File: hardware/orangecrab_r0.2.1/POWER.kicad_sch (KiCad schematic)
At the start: 43 parts, among them J5 JST, U1 TLV62569DRL, U10 NCP115-2.5, U2 TLV62569DRL, U5 BQ24232, U7 TLV62569DRL

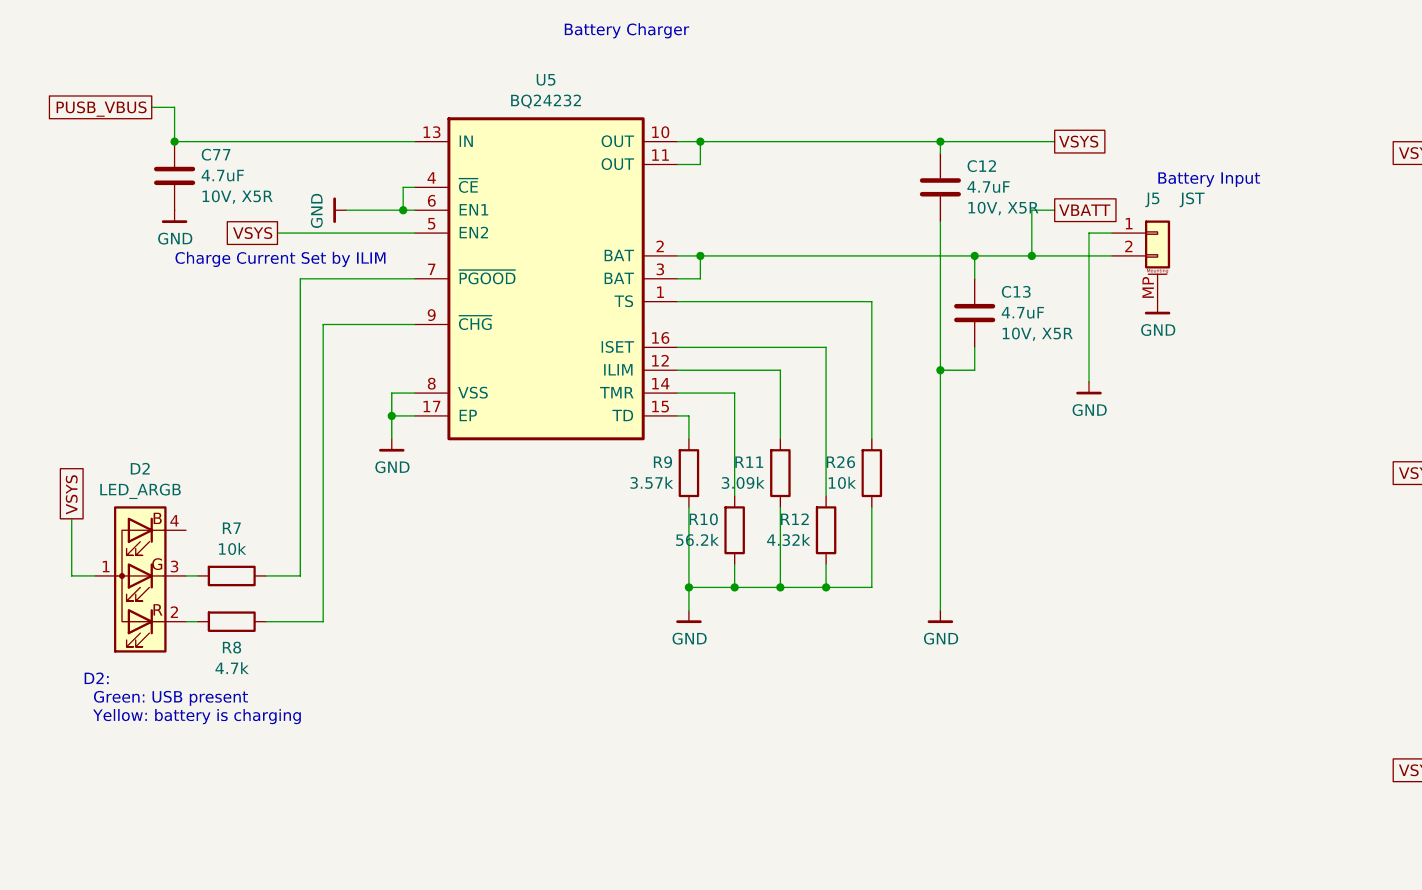
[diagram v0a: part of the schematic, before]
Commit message: all IO gone/cleaned
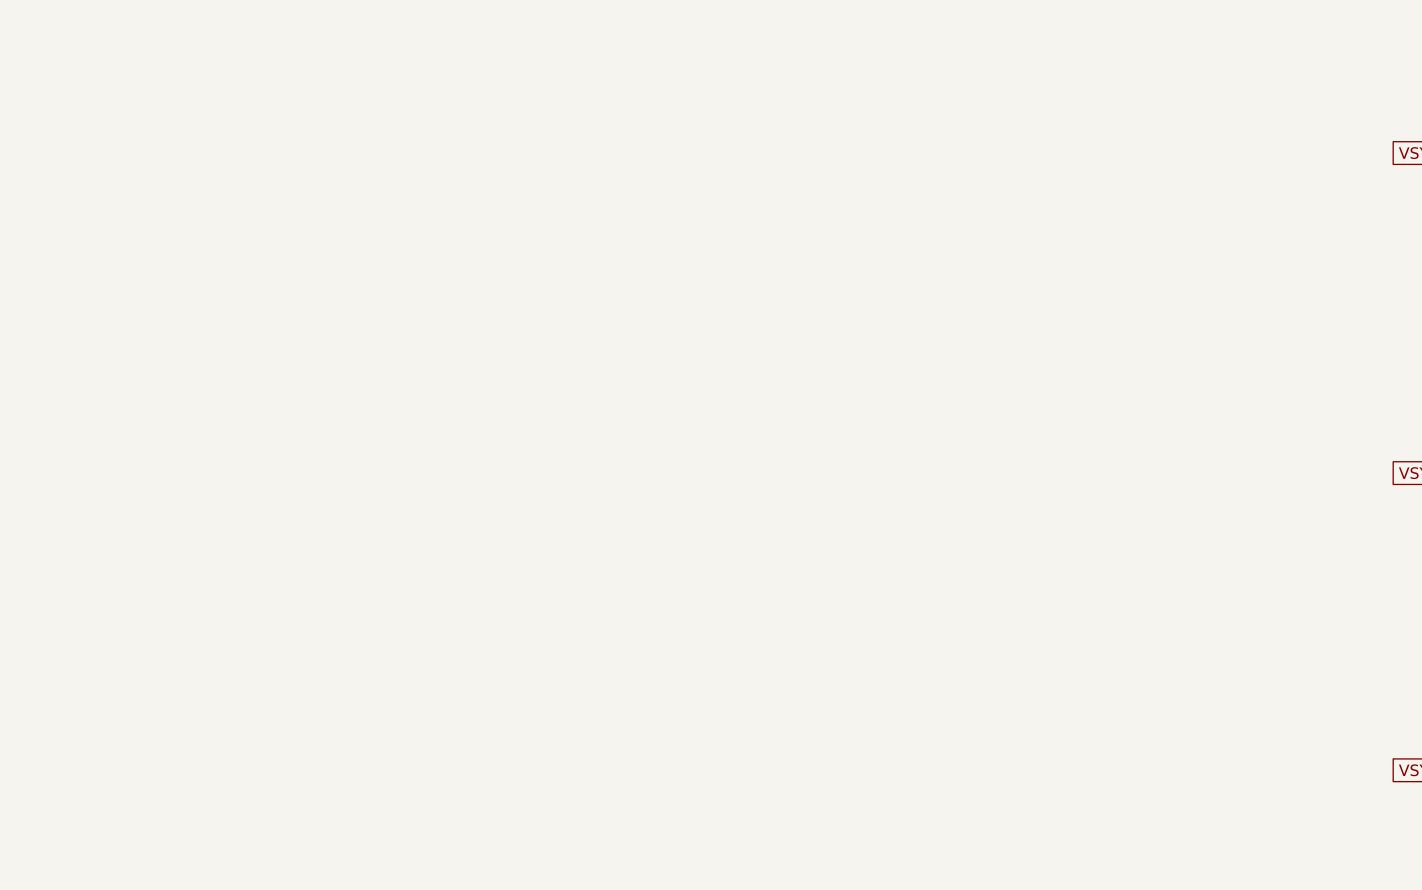
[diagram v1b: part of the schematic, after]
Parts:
- removed C12, C13, C77: 4.7uF, Capacitor_SMD:C_0402_1005Metric, symbol Device:C
- removed D2: LED_ARGB, gkl_led:0404LED_RGB, symbol Device:LED_ARGB
- removed J5: JST, gkl_conn:JST_PH_B2B-PH-SM4-TB_1x02-1MP_P2.00mm_Vertical, symbol Connector_Generic_MountingPin:Conn_01x02_MountingPin
- removed R10: 56.2k, gkl_dipol:R_0201_0603Metric, symbol Device:R
- removed R11: 3.09k, gkl_dipol:R_0201_0603Metric, symbol Device:R
- removed R12: 4.32k, gkl_dipol:R_0201_0603Metric, symbol Device:R
- removed R26, R7: 10k, gkl_dipol:R_0201_0603Metric, symbol Device:R
- removed R8: 4.7k, gkl_dipol:R_0201_0603Metric, symbol Device:R
- removed R9: 3.57k, gkl_dipol:R_0201_0603Metric, symbol Device:R
- removed U5: BQ24232, Package_DFN_QFN:QFN-16-1EP_3x3mm_P0.5mm_EP1.75x1.75mm, symbol gkl_pmic:BQ24230
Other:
- note removed: "Battery Charger"
- note removed: "Battery Input"
- note removed: "Charge Current Set by ILIM"
- note removed: "D2: Green: USB present Yellow: battery is charging"
